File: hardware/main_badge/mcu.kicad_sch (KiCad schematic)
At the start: 19 parts, among them U1 RP2350B, U2 W25Q128JVS, Y1 12MHz

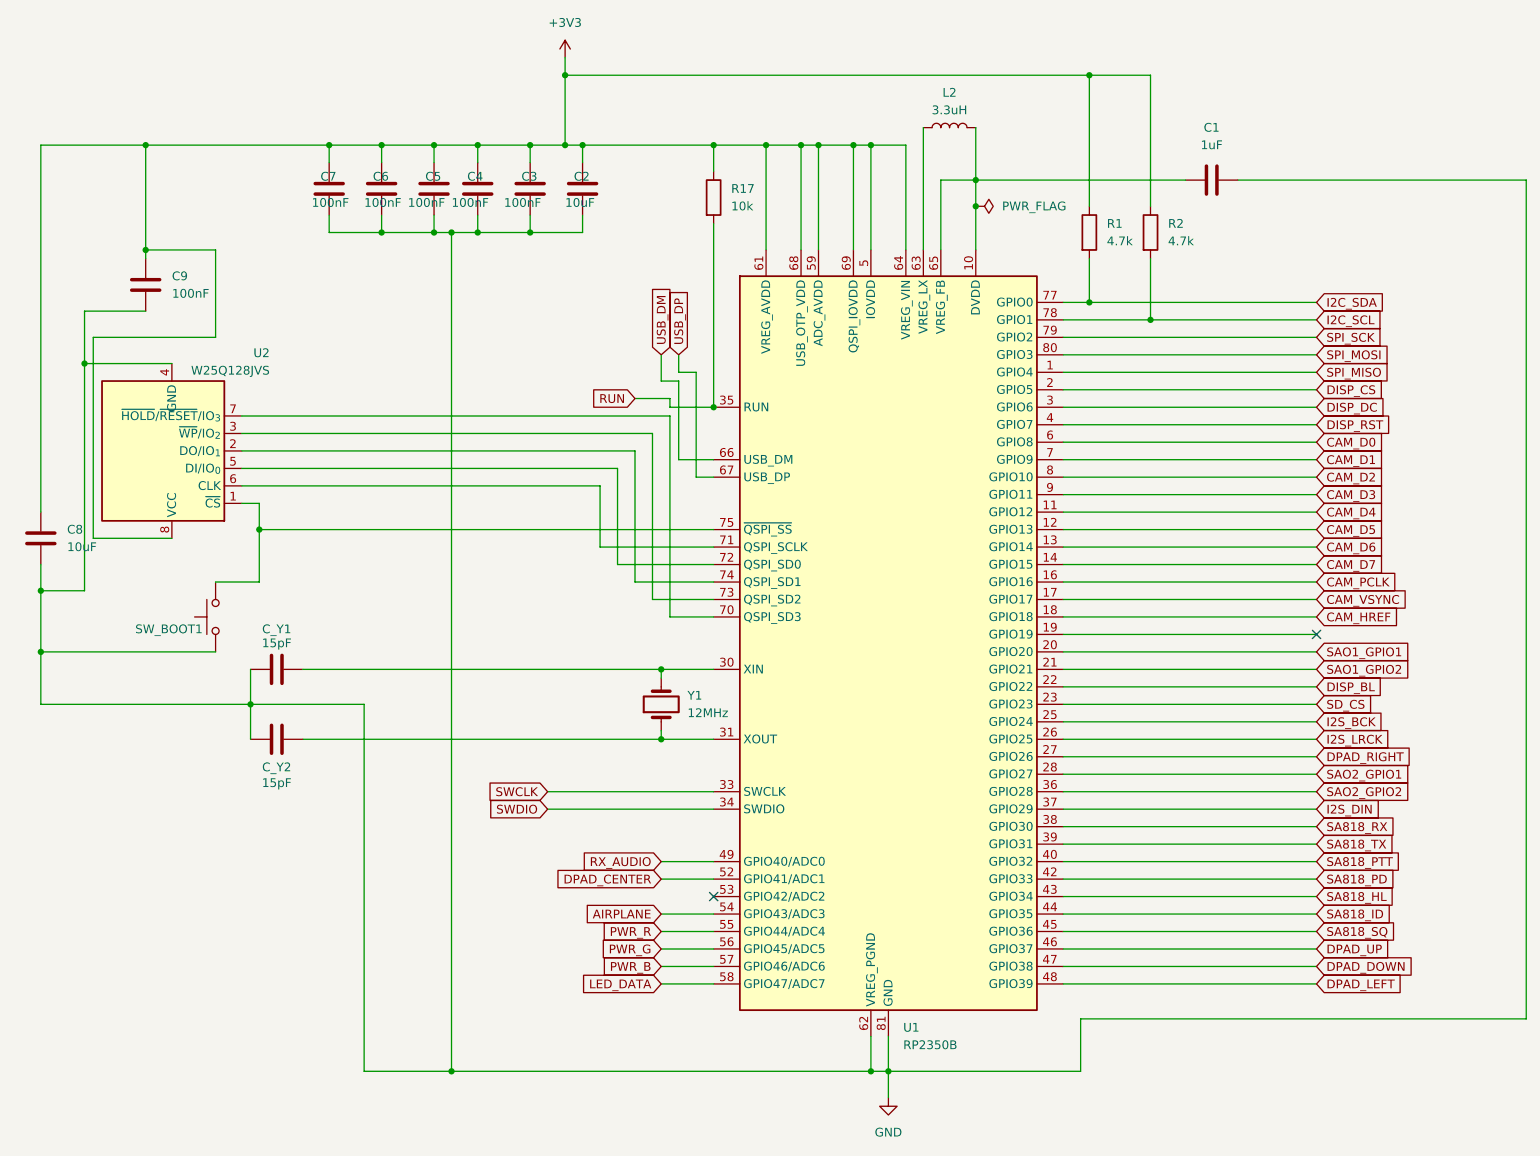
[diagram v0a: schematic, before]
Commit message: updated MCU pin layout
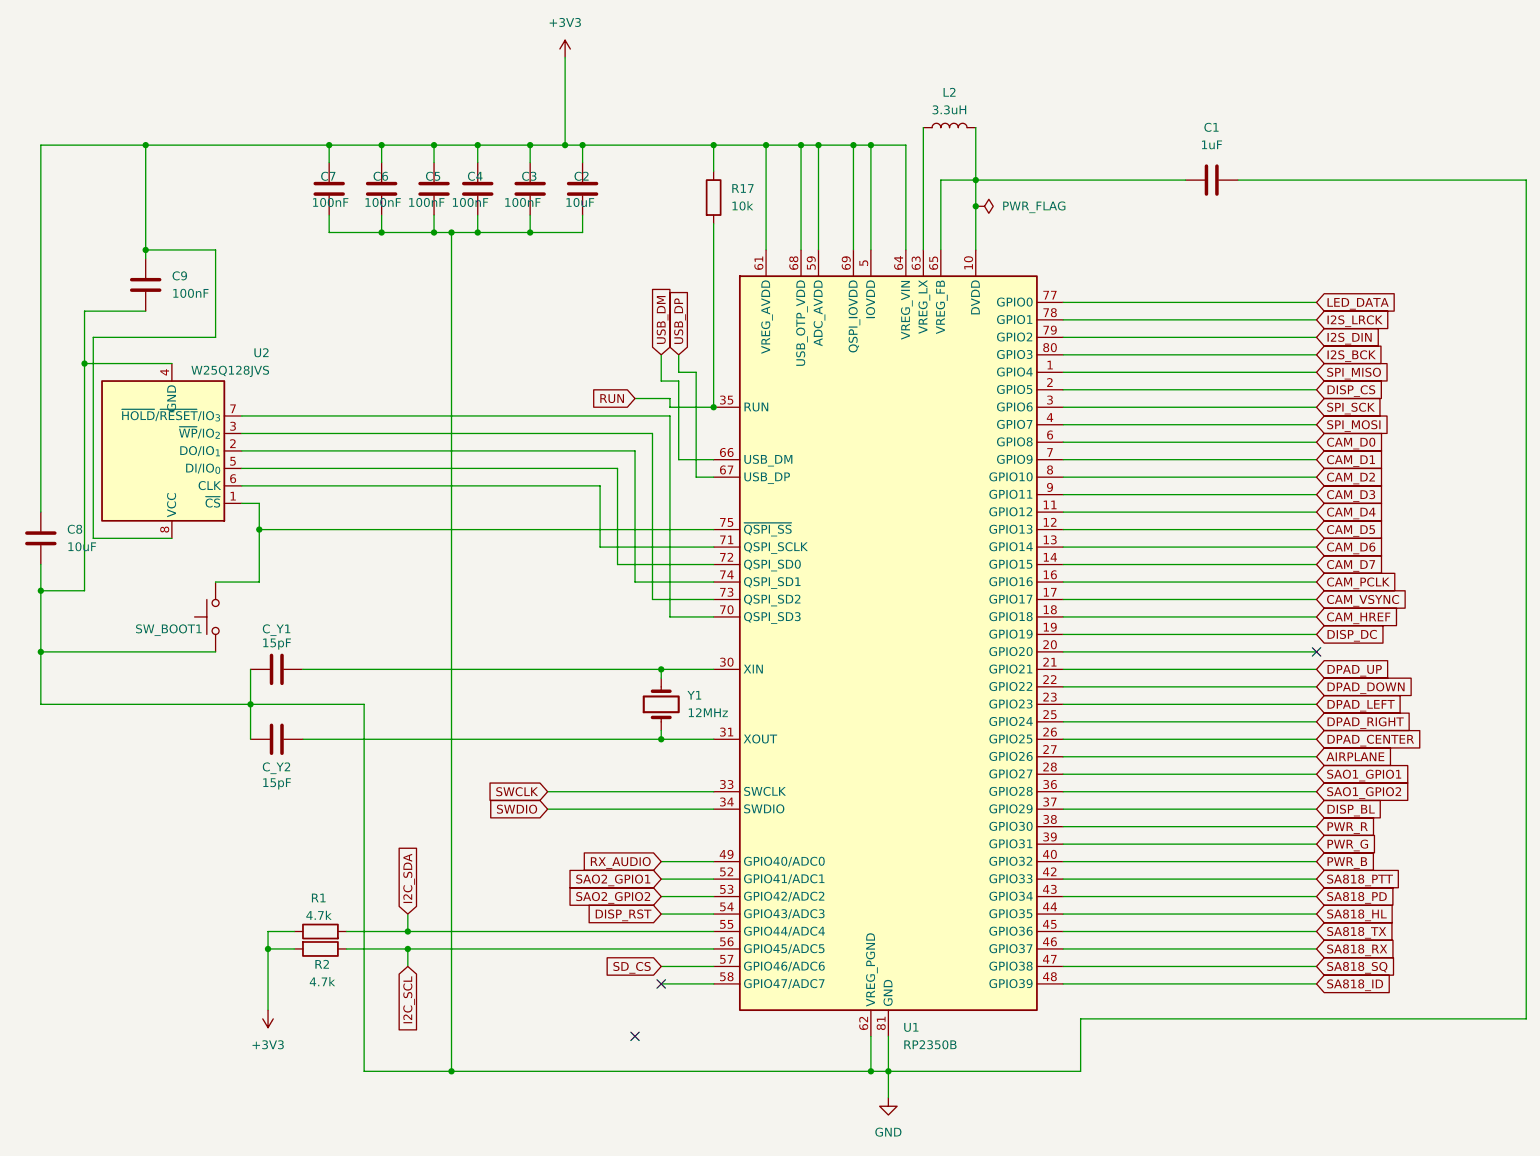
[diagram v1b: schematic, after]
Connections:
- net +3V3: now also R2.2; no longer R2.1
- net AIRPLANE: now also U1.27 (GPIO26); no longer U1.54 (GPIO43/ADC3)
- net DISP_BL: now also U1.37 (GPIO29); no longer U1.22 (GPIO22)
- net DISP_DC: now also U1.19 (GPIO19); no longer U1.3 (GPIO6)
- net DISP_RST: now also U1.54 (GPIO43/ADC3); no longer U1.4 (GPIO7)
- net DPAD_CENTER: now also U1.26 (GPIO25); no longer U1.52 (GPIO41/ADC1)
- net DPAD_DOWN: now also U1.22 (GPIO22); no longer U1.47 (GPIO38)
- net DPAD_LEFT: now also U1.23 (GPIO23); no longer U1.48 (GPIO39)
- net DPAD_RIGHT: now also U1.25 (GPIO24); no longer U1.27 (GPIO26)
- net DPAD_UP: now also U1.21 (GPIO21); no longer U1.46 (GPIO37)
- net I2C_SCL: now also R2.1, U1.56 (GPIO45/ADC5); no longer R2.2, U1.78 (GPIO1)
- net I2C_SDA: now also U1.55 (GPIO44/ADC4); no longer U1.77 (GPIO0)
- net I2S_BCK: now also U1.80 (GPIO3); no longer U1.25 (GPIO24)
- net I2S_DIN: now also U1.79 (GPIO2); no longer U1.37 (GPIO29)
- net I2S_LRCK: now also U1.78 (GPIO1); no longer U1.26 (GPIO25)
- net LED_DATA: now also U1.77 (GPIO0); no longer U1.58 (GPIO47/ADC7)
- net PWR_B: now also U1.40 (GPIO32); no longer U1.57 (GPIO46/ADC6)
- net PWR_G: now also U1.39 (GPIO31); no longer U1.56 (GPIO45/ADC5)
- net PWR_R: now also U1.38 (GPIO30); no longer U1.55 (GPIO44/ADC4)
- net SA818_HL: now also U1.44 (GPIO35); no longer U1.43 (GPIO34)
- net SA818_ID: now also U1.48 (GPIO39); no longer U1.44 (GPIO35)
- net SA818_PD: now also U1.43 (GPIO34); no longer U1.42 (GPIO33)
- net SA818_PTT: now also U1.42 (GPIO33); no longer U1.40 (GPIO32)
- net SA818_RX: now also U1.46 (GPIO37); no longer U1.38 (GPIO30)
- net SA818_SQ: now also U1.47 (GPIO38); no longer U1.45 (GPIO36)
- net SA818_TX: now also U1.45 (GPIO36); no longer U1.39 (GPIO31)
- net SAO1_GPIO1: now also U1.28 (GPIO27); no longer U1.20 (GPIO20)
- net SAO1_GPIO2: now also U1.36 (GPIO28); no longer U1.21 (GPIO21)
- net SAO2_GPIO1: now also U1.52 (GPIO41/ADC1); no longer U1.28 (GPIO27)
- net SAO2_GPIO2: now also U1.53 (GPIO42/ADC2); no longer U1.36 (GPIO28)
- net SD_CS: now also U1.57 (GPIO46/ADC6); no longer U1.23 (GPIO23)
- net SPI_MOSI: now also U1.4 (GPIO7); no longer U1.80 (GPIO3)
- net SPI_SCK: now also U1.3 (GPIO6); no longer U1.79 (GPIO2)
- no-connect marks 2 -> 3
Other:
- moved on the sheet: R1, R2

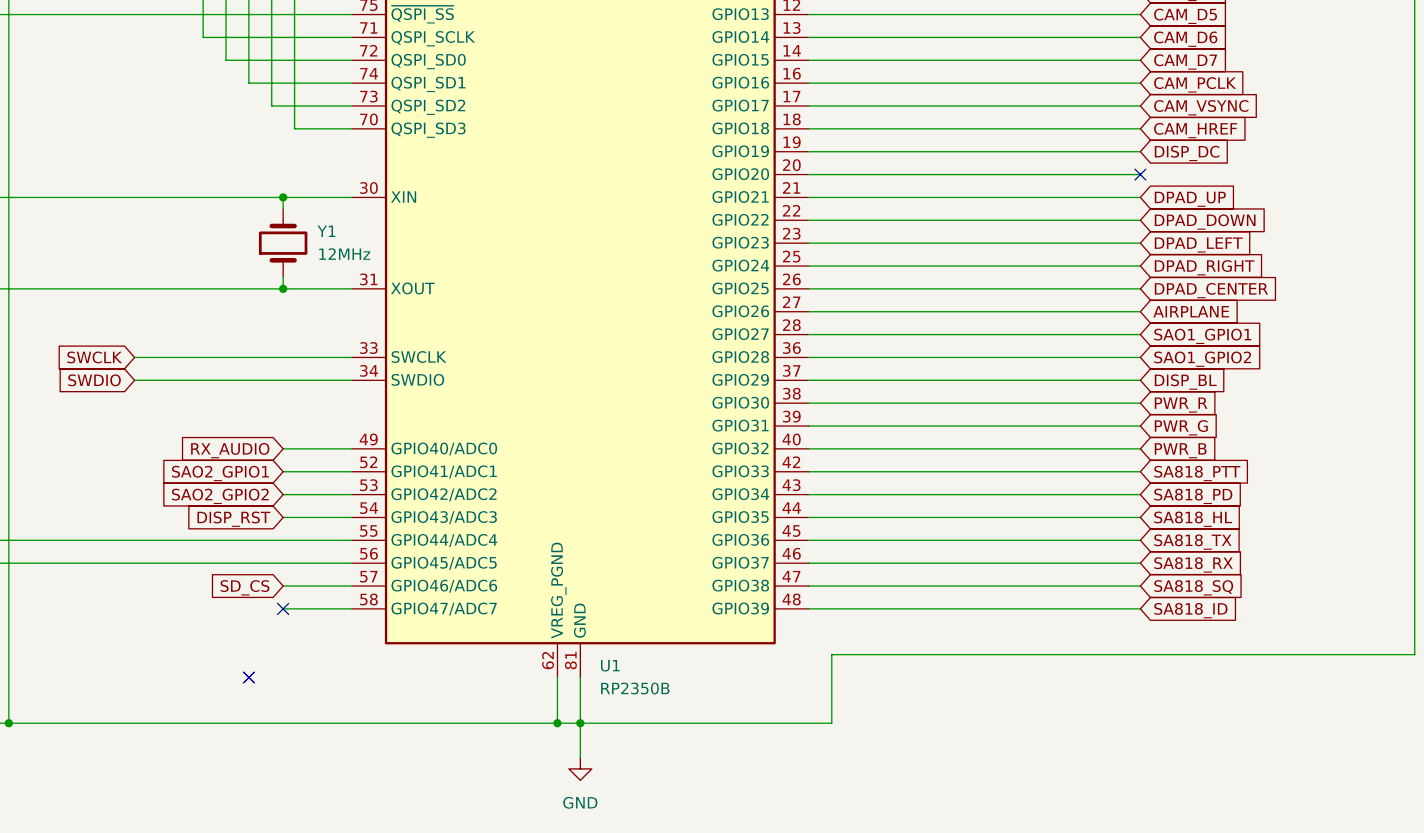
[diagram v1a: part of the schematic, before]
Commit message: wip routing
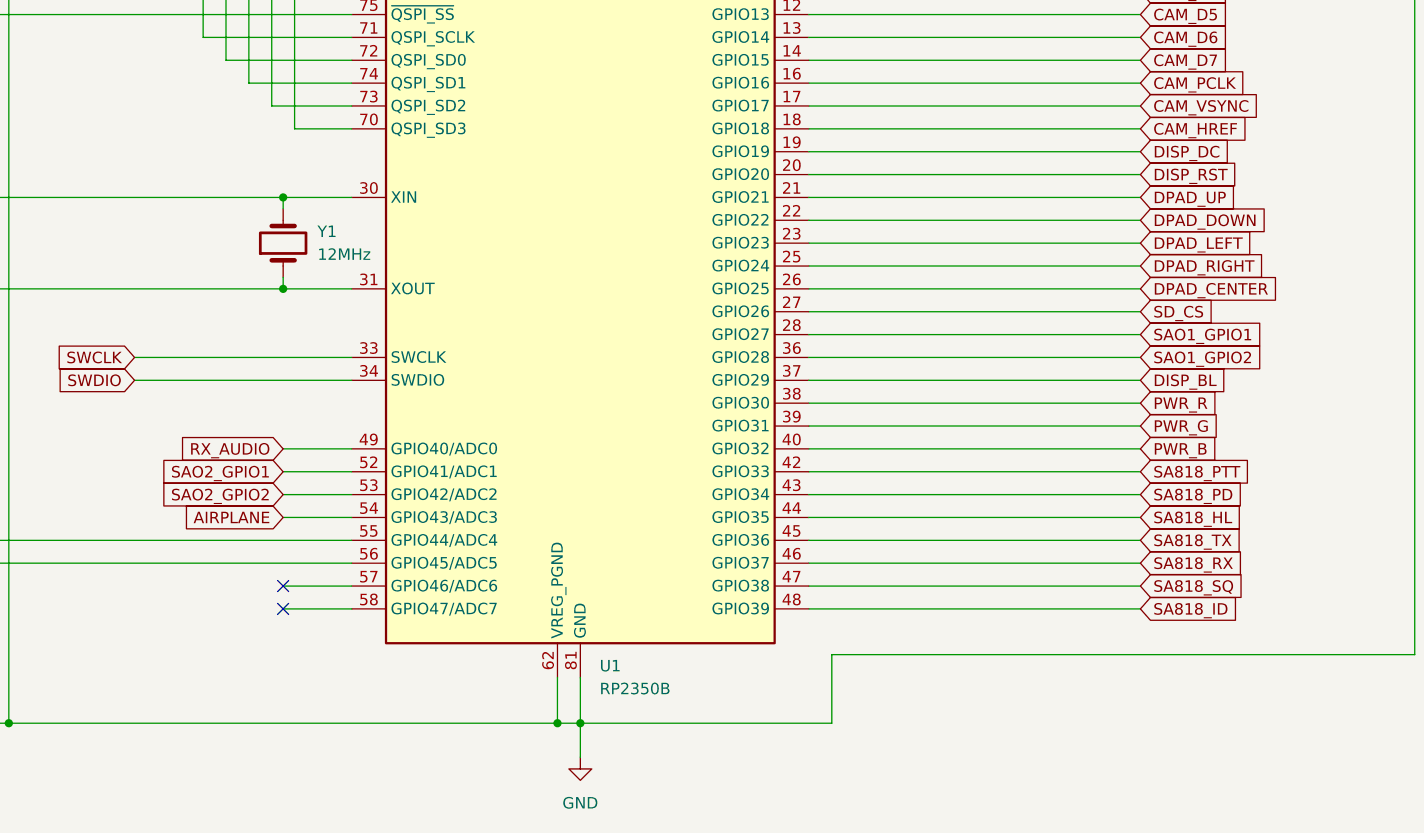
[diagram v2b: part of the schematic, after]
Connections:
- net AIRPLANE: now also U1.54 (GPIO43/ADC3); no longer U1.27 (GPIO26)
- net DISP_RST: now also U1.20 (GPIO20); no longer U1.54 (GPIO43/ADC3)
- net SD_CS: now also U1.27 (GPIO26); no longer U1.57 (GPIO46/ADC6)
- no-connect marks 3 -> 2
